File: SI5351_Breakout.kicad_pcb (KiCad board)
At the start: 2 copper layers, 139.7 x 42.5 mm, 33 parts, among them J1 Conn_01x03_Female, J10 Conn_01x02_Female, J17 CON-SMA-EDGE-S, J18 CON-SMA-EDGE-S, J19 CON-SMA-EDGE-S, J2 Conn_01x02_Female, J3 Conn_01x02_Female, J4 Conn_01x02_Female, J5 Conn_01x02_Female, J6 Conn_01x02_Female, J7 Conn_01x02_Female, J8 Conn_01x02_Female, J9 Conn_01x02_Female, K1 G5V-2, K2 G5V-2, K3 G5V-2, U1 AMP, U2 AMP, U3 AMP

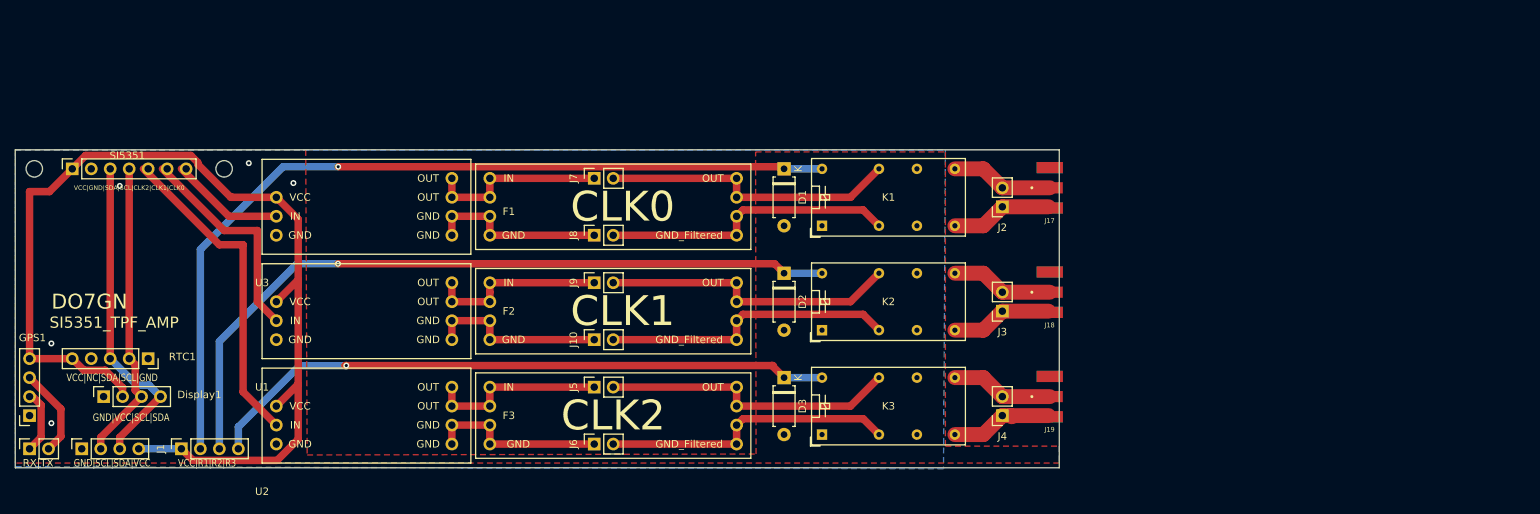
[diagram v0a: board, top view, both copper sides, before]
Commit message: latest version
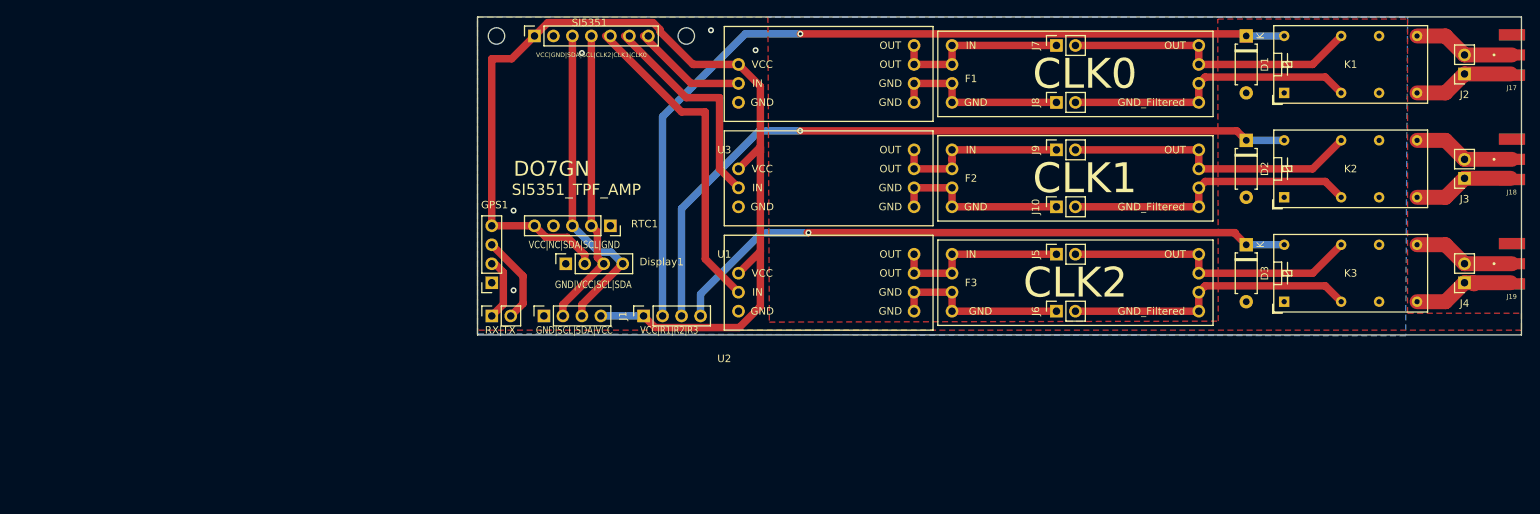
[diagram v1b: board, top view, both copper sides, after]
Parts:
- moved F1 64.4 mm to (148.7, 40.1)
- moved F2 64.4 mm to (148.7, 54.1)
- moved F3 64.4 mm to (148.7, 68.1)
- moved J10 64.4 mm to (162.7, 64.3)
- moved J5 64.4 mm to (162.7, 70.6)
- moved J6 64.4 mm to (162.7, 78.2)
- moved J7 64.4 mm to (162.7, 42.7)
- moved J8 64.4 mm to (162.7, 50.3)
- moved J9 64.4 mm to (162.7, 56.6)
- moved Display1 64.4 mm to (97.0, 71.9)
- moved GPS1 64.4 mm to (87.1, 74.4)
- moved REF** 64.4 mm to (87.8, 41.4)
- moved RX|TX 64.4 mm to (87.1, 78.9)
- moved SI5351 64.4 mm to (92.8, 41.4)
- moved Arduino1 64.4 mm to (94.1, 78.9)
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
